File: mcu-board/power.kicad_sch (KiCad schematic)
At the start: 15 parts, among them Q1 SSM3J328R,LF, Q2 SSM3J328R,LF, U2 L7806, U3 L7806, U4 AZ1117-3.3

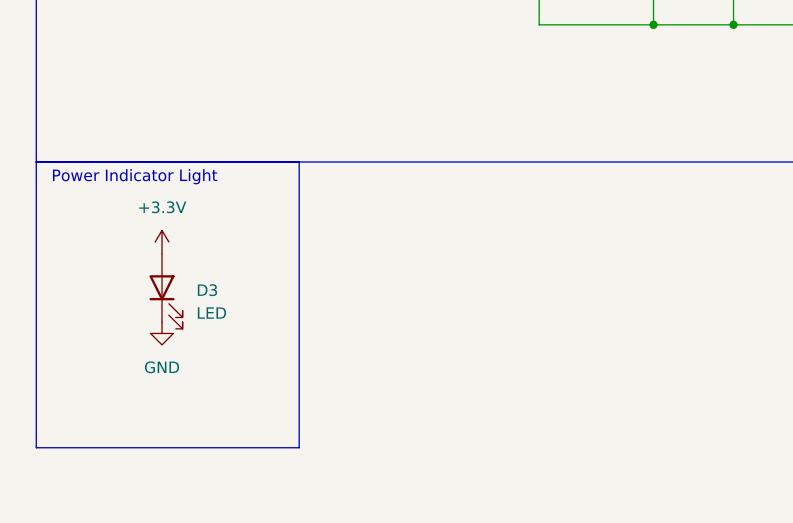
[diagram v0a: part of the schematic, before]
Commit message: finished schematic(?)
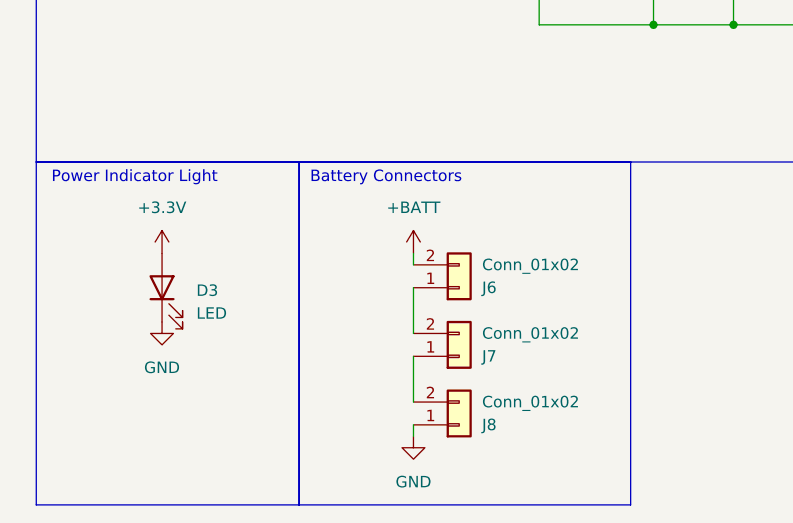
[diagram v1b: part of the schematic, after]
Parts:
- added J6, J7, J8: Conn_01x02, Connector_JST:JST_PH_B2B-PH-K_1x02_P2.00mm_Vertical, symbol Connector_Generic:Conn_01x02
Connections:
- net +BATT: now also J6.2 (Pin_2)
- net GND: now also J8.1 (Pin_1)
- new net: J6.1 (Pin_1), J7.2 (Pin_2)
- new net: J7.1 (Pin_1), J8.2 (Pin_2)
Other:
- note added: "Battery Connectors"

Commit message: footprints
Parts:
- C1, C2, C3, C4: footprint Capacitor_SMD:C_1206_3216Metric -> Capacitor_SMD:C_0603_1608Metric
- C5, C6: footprint Capacitor_SMD:C_1206_3216Metric -> Capacitor_SMD:C_0805_2012Metric
- R3: footprint Resistor_SMD:R_1206_3216Metric -> Resistor_SMD:R_0603_1608Metric
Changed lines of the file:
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@@
 		(dnp no)
 		(fields_autoplaced yes)
-		(property "Reference" "#PWR?"
+		(property "Reference" "#PWR0107"
 			(at 124.46 82.55 0)
 			(effects
@@
 			(project "mcu board"
 				(path "/e926887c-cd26-4f47-be51-3352b14f6743/65b6e221-2db7-4e52-96fb-70ae76f49758"
-					(reference "#PWR?")
+					(reference "#PWR0107")
 					(unit 1)
 				)
@@
 		(dnp no)
 		(fields_autoplaced yes)
-		(property "Reference" "#PWR?"
+		(property "Reference" "#PWR0102"
 			(at 187.96 82.55 0)
 			(effects
@@
 			(project "mcu board"
 				(path "/e926887c-cd26-4f47-be51-3352b14f6743/65b6e221-2db7-4e52-96fb-70ae76f49758"
-					(reference "#PWR?")
+					(reference "#PWR0102")
 					(unit 1)
 				)
@@
 			)
 		)
-		(property "Footprint" "Capacitor_SMD:C_1206_3216Metric"
+		(property "Footprint" "Capacitor_SMD:C_0603_1608Metric"
 			(at 116.84 90.17 0)
 			(effects
@@
 		(dnp no)
 		(fields_autoplaced yes)
-		(property "Reference" "#PWR?"
+		(property "Reference" "#PWR0103"
 			(at 179.07 133.35 0)
 			(effects
@@
 			(project "mcu board"
 				(path "/e926887c-cd26-4f47-be51-3352b14f6743/65b6e221-2db7-4e52-96fb-70ae76f49758"
-					(reference "#PWR?")
+					(reference "#PWR0103")
 					(unit 1)
 				)
@@
 		(dnp no)
 		(fields_autoplaced yes)
-		(property "Reference" "#PWR?"
+		(property "Reference" "#PWR0112"
 			(at 264.16 82.55 0)
 			(effects
@@
 			(project "mcu board"
 				(path "/e926887c-cd26-4f47-be51-3352b14f6743/65b6e221-2db7-4e52-96fb-70ae76f49758"
-					(reference "#PWR?")
+					(reference "#PWR0112")
 					(unit 1)
 				)
@@
 		(dnp no)
 		(fields_autoplaced yes)
-		(property "Reference" "#PWR?"
+		(property "Reference" "#PWR0110"
 			(at 209.55 133.35 0)
 			(effects
@@
 			(project "mcu board"
 				(path "/e926887c-cd26-4f47-be51-3352b14f6743/65b6e221-2db7-4e52-96fb-70ae76f49758"
-					(reference "#PWR?")
+					(reference "#PWR0110")
 					(unit 1)
 				)
@@
 		(dnp no)
 		(fields_autoplaced yes)
-		(property "Reference" "#PWR?"
+		(property "Reference" "#PWR0101"
 			(at 139.7 82.55 0)
 			(effects
@@
 			(project "mcu board"
 				(path "/e926887c-cd26-4f47-be51-3352b14f6743/65b6e221-2db7-4e52-96fb-70ae76f49758"
-					(reference "#PWR?")
+					(reference "#PWR0101")
 					(unit 1)
 				)
@@
 		(dnp no)
 		(fields_autoplaced yes)
-		(property "Reference" "#PWR?"
+		(property "Reference" "#PWR0111"
 			(at 276.86 82.55 0)
 			(effects
@@
 			(project "mcu board"
 				(path "/e926887c-cd26-4f47-be51-3352b14f6743/65b6e221-2db7-4e52-96fb-70ae76f49758"
-					(reference "#PWR?")
+					(reference "#PWR0111")
 					(unit 1)
 				)
@@
 			)
 		)
-		(property "Footprint" "Capacitor_SMD:C_1206_3216Metric"
+		(property "Footprint" "Capacitor_SMD:C_0603_1608Metric"
 			(at 116.84 115.57 0)
 			(effects
@@
 			)
 		)
-		(property "Footprint" "Capacitor_SMD:C_1206_3216Metric"
+		(property "Footprint" "Capacitor_SMD:C_0603_1608Metric"
 			(at 73.66 90.17 0)
 			(effects
@@
 		(dnp no)
 		(fields_autoplaced yes)
-		(property "Reference" "#PWR?"
+		(property "Reference" "#PWR0108"
 			(at 228.6 82.55 0)
 			(effects
@@
 			(project "mcu board"
 				(path "/e926887c-cd26-4f47-be51-3352b14f6743/65b6e221-2db7-4e52-96fb-70ae76f49758"
-					(reference "#PWR?")
+					(reference "#PWR0108")
 					(unit 1)
 				)
@@
 		(dnp no)
 		(fields_autoplaced yes)
-		(property "Reference" "#PWR?"
+		(property "Reference" "#PWR0106"
 			(at 114.3 133.35 0)
 			(effects
@@
 			(project "mcu board"
 				(path "/e926887c-cd26-4f47-be51-3352b14f6743/65b6e221-2db7-4e52-96fb-70ae76f49758"
-					(reference "#PWR?")
+					(reference "#PWR0106")
 					(unit 1)
 				)
@@
 			)
 		)
-		(property "Footprint" "Resistor_SMD:R_1206_3216Metric"
+		(property "Footprint" "Resistor_SMD:R_0603_1608Metric"
 			(at 209.55 97.79 0)
 			(effects
@@
 			)
 		)
-		(property "Footprint" "Capacitor_SMD:C_1206_3216Metric"
+		(property "Footprint" "Capacitor_SMD:C_0603_1608Metric"
 			(at 73.66 115.57 0)
 			(effects
@@
 			)
 		)
-		(property "Footprint" "Capacitor_SMD:C_1206_3216Metric"
+		(property "Footprint" "Capacitor_SMD:C_0805_2012Metric"
 			(at 147.32 90.17 0)
 			(effects
@@
 		(dnp no)
 		(fields_autoplaced yes)
-		(property "Reference" "#PWR?"
+		(property "Reference" "#PWR0104"
 			(at 24.13 82.55 0)
 			(effects
@@
 			(project "mcu board"
 				(path "/e926887c-cd26-4f47-be51-3352b14f6743/65b6e221-2db7-4e52-96fb-70ae76f49758"
-					(reference "#PWR?")
+					(reference "#PWR0104")
 					(unit 1)
 				)
@@
 		(dnp no)
 		(fields_autoplaced yes)
-		(property "Reference" "#PWR?"
+		(property "Reference" "#PWR0105"
 			(at 46.99 82.55 0)
 			(effects
@@
 			(project "mcu board"
 				(path "/e926887c-cd26-4f47-be51-3352b14f6743/65b6e221-2db7-4e52-96fb-70ae76f49758"
-					(reference "#PWR?")
+					(reference "#PWR0105")
 					(unit 1)
 				)
@@
 		(dnp no)
 		(fields_autoplaced yes)
-		(property "Reference" "#PWR?"
+		(property "Reference" "#PWR0109"
 			(at 242.57 82.55 0)
 			(effects
@@
 			(project "mcu board"
 				(path "/e926887c-cd26-4f47-be51-3352b14f6743/65b6e221-2db7-4e52-96fb-70ae76f49758"
-					(reference "#PWR?")
+					(reference "#PWR0109")
 					(unit 1)
 				)
@@
 			)
 		)
-		(property "Footprint" "Capacitor_SMD:C_1206_3216Metric"
+		(property "Footprint" "Capacitor_SMD:C_0805_2012Metric"
 			(at 179.07 90.17 0)
 			(effects
